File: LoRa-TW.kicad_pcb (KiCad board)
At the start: 4 copper layers, 15 x 26.6 mm, 47 parts, among them J1 MHF-I/U.FL, J2 Conn_02x06_2.0mm, J3 RFShield_OnePiece, U1 SX1262IMLTRT, X1 TCXO, 32MHz, 2.0x1.6mm

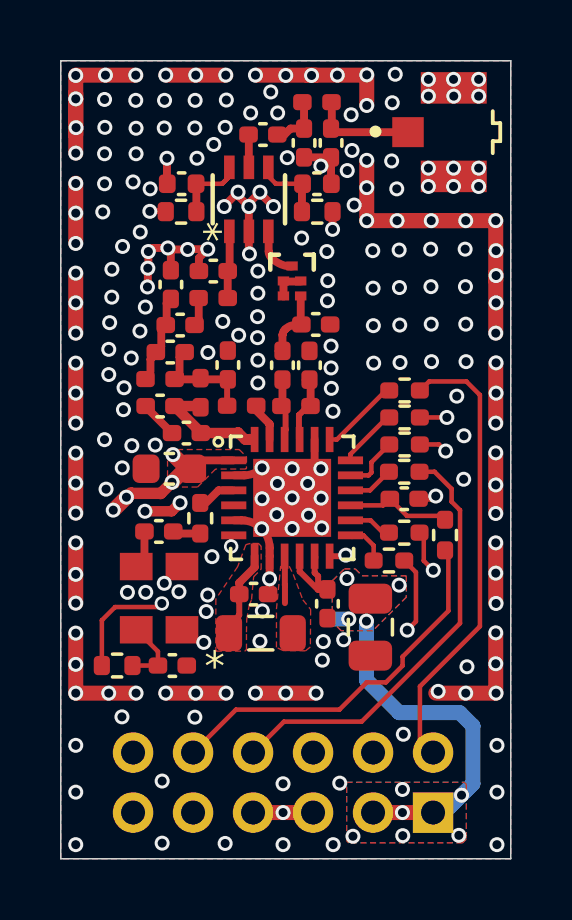
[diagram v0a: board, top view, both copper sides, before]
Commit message: prepare for BOM generation
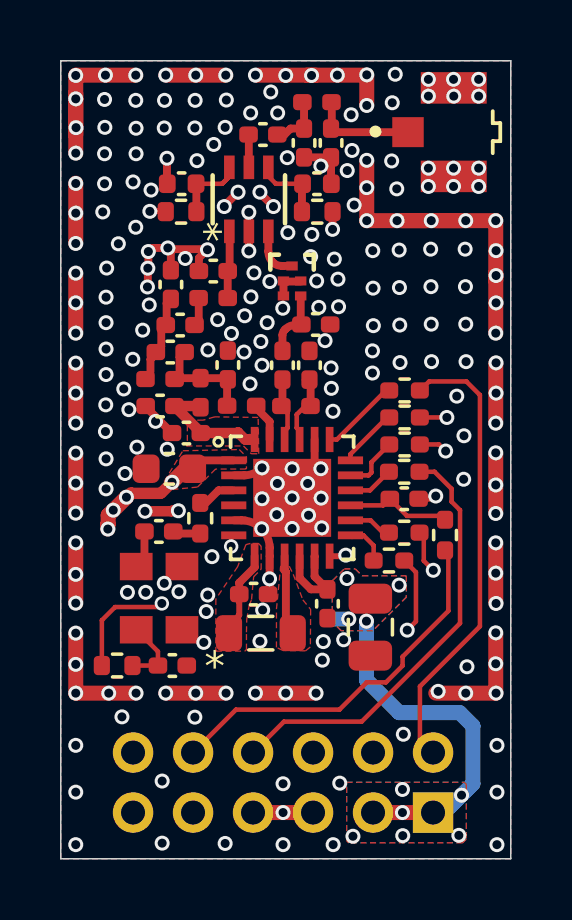
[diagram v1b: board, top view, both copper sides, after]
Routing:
- net GND: track 23.1 -> 21.6 mm, vias 222 -> 234
- net Net-(U1-DCC_SW): track 1.57 -> 2.70 mm
- net VDD: track 42.6 -> 41.6 mm
- added copper zone on F.Cu, net Net-(U1-VR_PA)
